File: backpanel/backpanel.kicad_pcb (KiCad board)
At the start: 2 copper layers, 8 parts

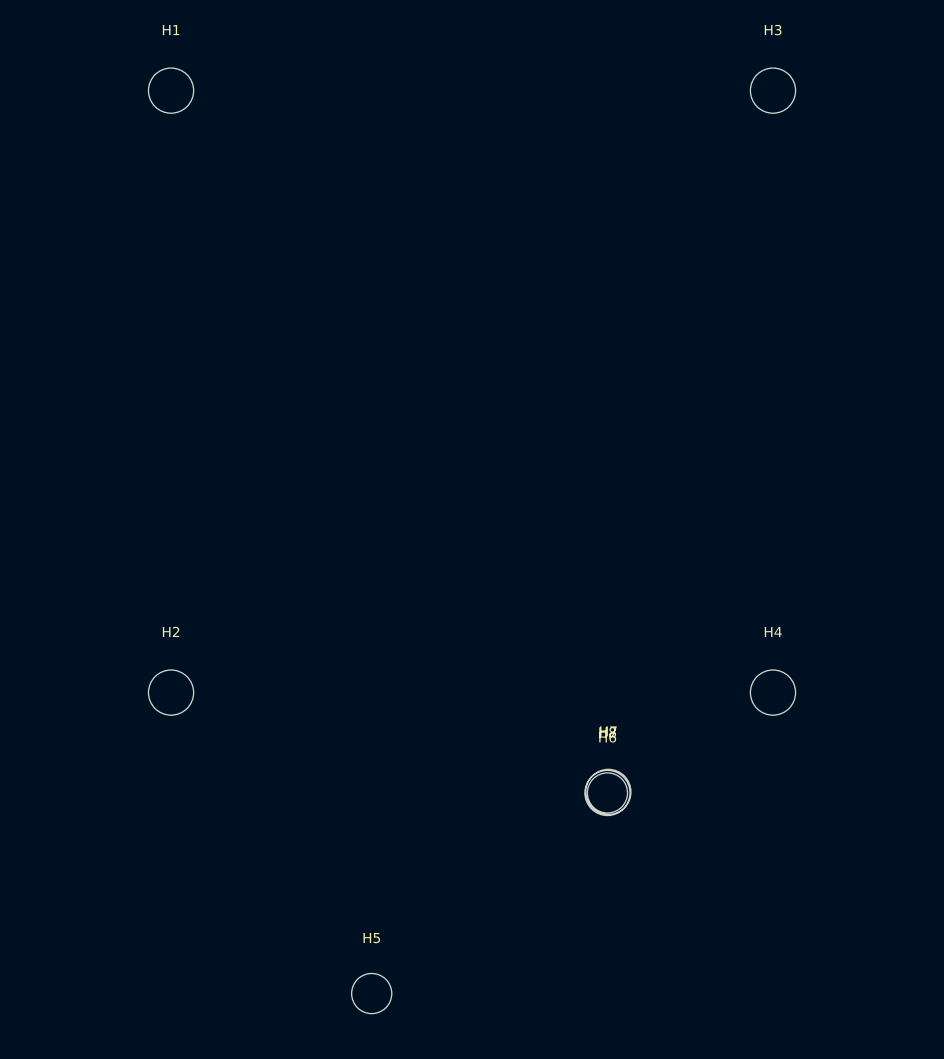
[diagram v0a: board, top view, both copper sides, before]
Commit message: added dfm changes from fab, I think
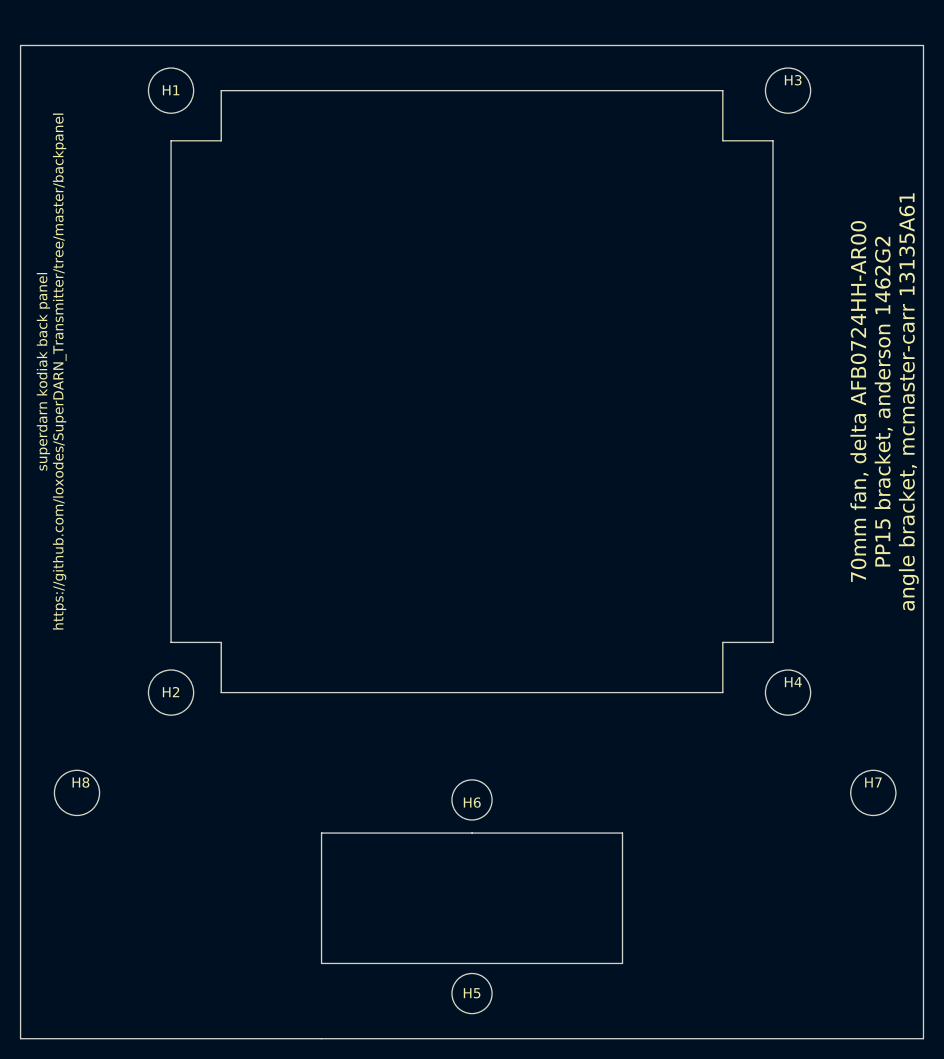
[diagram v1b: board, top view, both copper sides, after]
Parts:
- moved H8 52.9 mm to (95.6, 105.0)
- moved H7 26.4 mm to (175.0, 105.0)
- moved H6 13.5 mm to (135.0, 105.7)
- moved H5 10.0 mm to (135.0, 125.0)
- moved H3 1.50 mm to (166.5, 35.0)
- moved H4 1.50 mm to (166.5, 95.0)
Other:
- board outline added: 90 x 99 mm
- board text added: "70mm fan, delta AFB0724HH-AR00 PP15 bracket, anderson 1462G2 angle bracket, mcmaster-carr 13135A61"
- board text added: "superdarn kodiak back panel https://github.com/loxodes/SuperDARN_Transmitter/tree/master/backpanel"
